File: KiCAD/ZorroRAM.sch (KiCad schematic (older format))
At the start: 19 parts, among them J1 Conn_01x06_Male, U2 AP2210N-3.3TRG1, U3 74LVC245, U4 74LVC245, U5 XC9572XL-10VQ64C, U6 K4E641612D

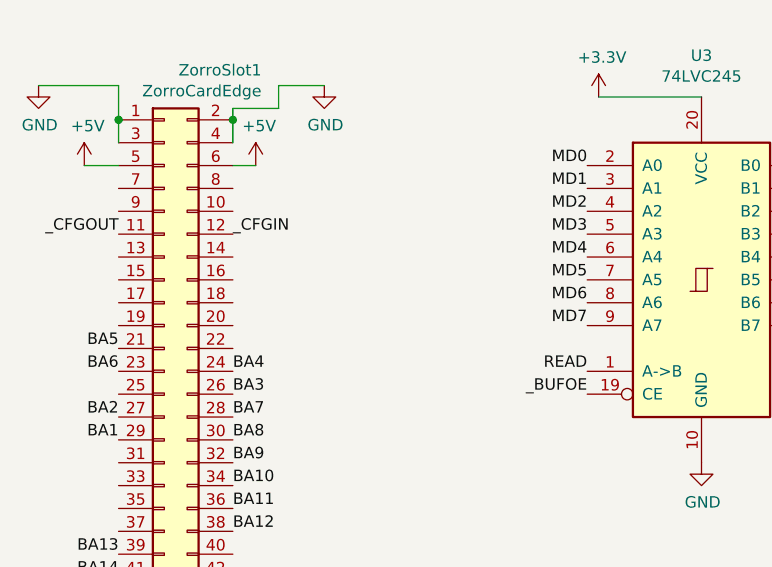
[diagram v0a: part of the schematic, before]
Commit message: Add files via upload
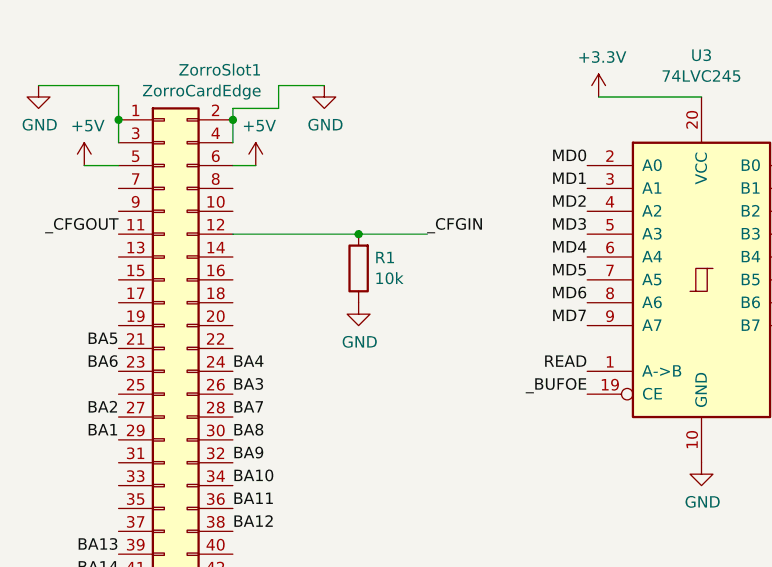
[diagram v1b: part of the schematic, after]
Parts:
- added R1: 10k, Resistor_SMD:R_1206_3216Metric, symbol Device:R
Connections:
- net GND: now also R1.1
- net _CFGIN: now also R1.2
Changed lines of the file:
@@
 Text Label 1700 6150 0    50   ~ 0
 E7M
-Text Label 1700 2150 0    50   ~ 0
+Text Label 2550 2150 0    50   ~ 0
 _CFGIN
 Text Label 1200 2150 2    50   ~ 0
@@
 	1200 6750 1450 6750
 Connection ~ 1450 6750
+$Comp
+L Device:R R1
+U 1 1 60BC61F6
+P 2250 2300
+F 0 "R1" H 2180 2254 50  0000 R CNN
+F 1 "10k" H 2180 2345 50  0000 R CNN
+F 2 "Resistor_SMD:R_1206_3216Metric" V 2180 2300 50  0001 C CNN
+F 3 "~" H 2250 2300 50  0001 C CNN
+	1    2250 2300
+	-1   0    0    1
+$EndComp
+Wire Wire Line
+	2550 2150 2250 2150
+Connection ~ 2250 2150
+Wire Wire Line
+	2250 2150 1700 2150
+$Comp
+L power:GND #PWR?
+U 1 1 60BDABC6
+P 2250 2450
+F 0 "#PWR?" H 2250 2200 50  0001 C CNN
+F 1 "GND" H 2255 2277 50  0000 C CNN
+F 2 "" H 2250 2450 50  0001 C CNN
+F 3 "" H 2250 2450 50  0001 C CNN
+	1    2250 2450
+	1    0    0    -1
+$EndComp
 $EndSCHEMATC

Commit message: Add files via upload
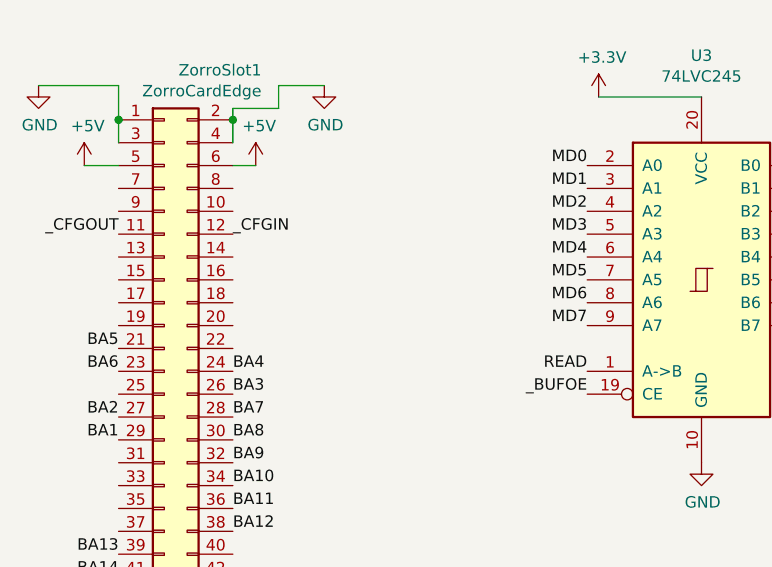
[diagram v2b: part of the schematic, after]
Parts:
- removed R1: 10k, Resistor_SMD:R_1206_3216Metric, symbol Device:R
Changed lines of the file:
@@
 Text Label 1700 6150 0    50   ~ 0
 E7M
-Text Label 2550 2150 0    50   ~ 0
+Text Label 1700 2150 0    50   ~ 0
 _CFGIN
 Text Label 1200 2150 2    50   ~ 0
@@
 	1200 6750 1450 6750
 Connection ~ 1450 6750
-$Comp
-L Device:R R1
-U 1 1 60BC61F6
-P 2250 2300
-F 0 "R1" H 2180 2254 50  0000 R CNN
-F 1 "10k" H 2180 2345 50  0000 R CNN
-F 2 "Resistor_SMD:R_1206_3216Metric" V 2180 2300 50  0001 C CNN
-F 3 "~" H 2250 2300 50  0001 C CNN
-	1    2250 2300
-	-1   0    0    1
-$EndComp
-Wire Wire Line
-	2550 2150 2250 2150
-Connection ~ 2250 2150
-Wire Wire Line
-	2250 2150 1700 2150
-$Comp
-L power:GND #PWR?
-U 1 1 60BDABC6
-P 2250 2450
-F 0 "#PWR?" H 2250 2200 50  0001 C CNN
-F 1 "GND" H 2255 2277 50  0000 C CNN
-F 2 "" H 2250 2450 50  0001 C CNN
-F 3 "" H 2250 2450 50  0001 C CNN
-	1    2250 2450
-	1    0    0    -1
-$EndComp
 $EndSCHEMATC
